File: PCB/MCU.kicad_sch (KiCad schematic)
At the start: 12 parts, among them J1 TC2030-NL, U7 STM32G431C8Ux

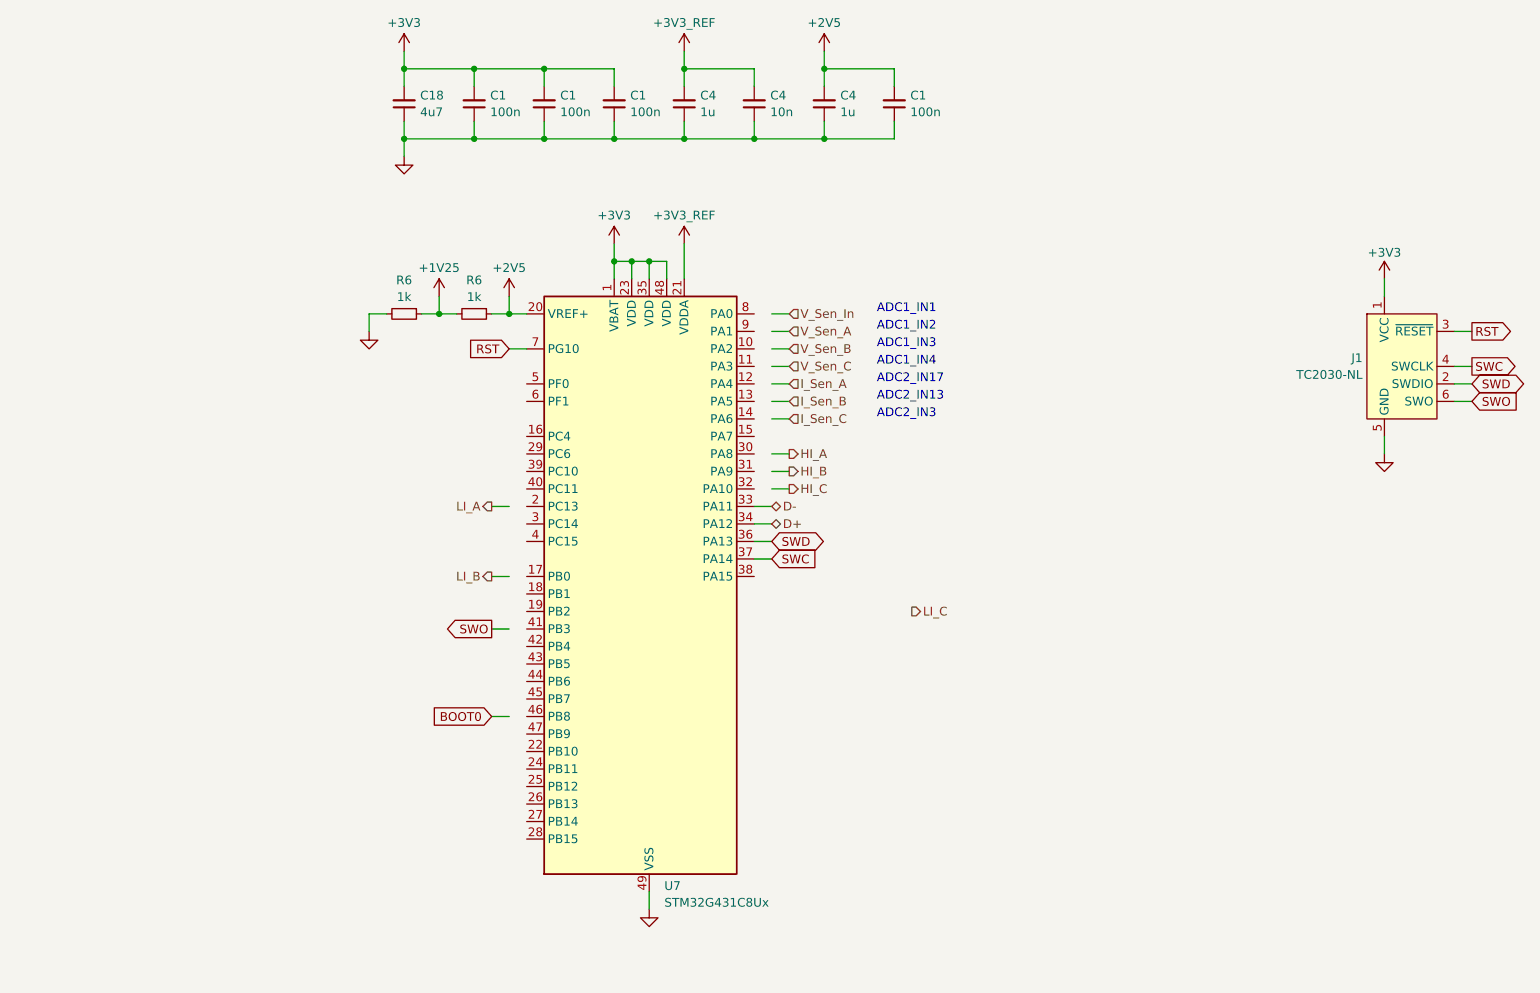
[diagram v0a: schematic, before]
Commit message: f
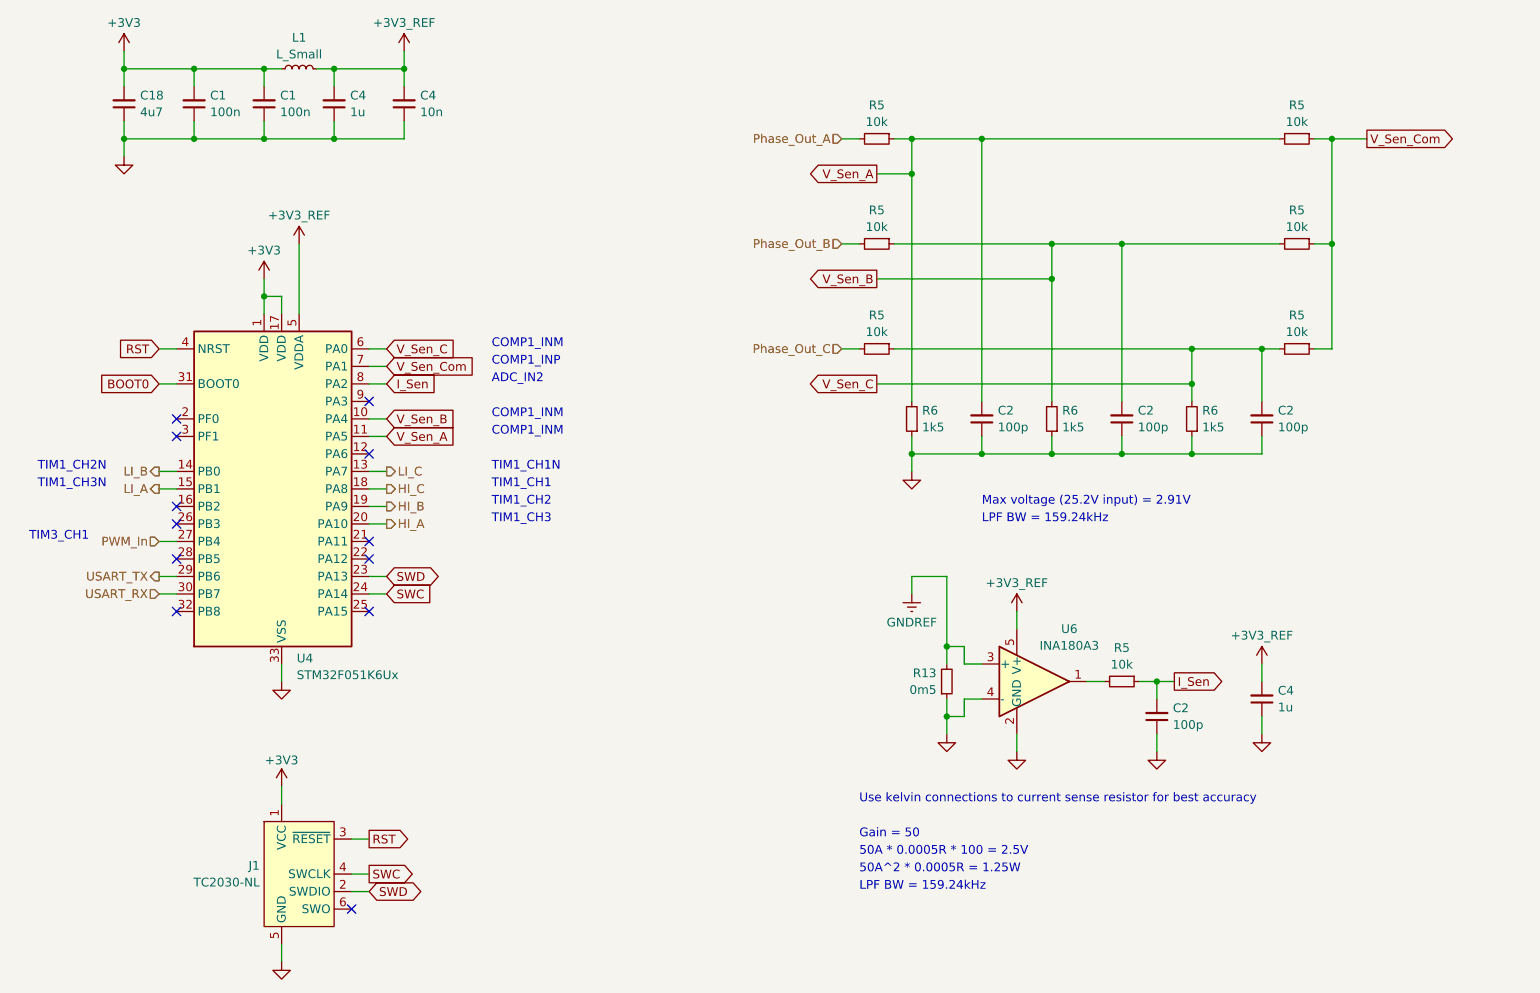
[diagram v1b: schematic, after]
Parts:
- removed C1 (x2): 100n, symbol Device:C_Small
- removed R6 (x2): 1k, symbol Device:R_Small
- removed U7: STM32G431C8Ux, Package_DFN_QFN:QFN-48-1EP_7x7mm_P0.5mm_EP5.6x5.6mm, symbol MCU_ST_STM32G4:STM32G431C8Ux
- added C2 (x4): 100p, symbol Device:C_Small
- added L1: L_Small, symbol Device:L_Small
- added R13: 0m5, symbol Device:R_Small
- added R5 (x7): 10k, symbol Device:R_Small
- added R6 (x3): 1k5, symbol Device:R_Small
- added U4: STM32F051K6Ux, Package_DFN_QFN:QFN-32-1EP_5x5mm_P0.5mm_EP3.45x3.45mm, symbol MCU_ST_STM32F0:STM32F051K6Ux
- added U6: INA180A3, Package_TO_SOT_SMD:SOT-23-5, symbol Amplifier_Current:INA180A3
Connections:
- net +2V5 is gone; now on net +3V3_REF: C4.2
- net +3V3: now also L1.1, U4.1 (VDD), U4.17 (VDD)
- net +3V3_REF: now also L1.2, U4.5 (VDDA), U6.5 (V+)
- net BOOT0: now also U4.31 (BOOT0)
- net GND: now also C2.1, C2.1, C2.1, C2.1, R13.1, R6.1, R6.1, R6.1, U4.33 (VSS), U6.2 (GND), U6.4 (-)
- net HI_A: now also U4.20 (PA10)
- net HI_B: now also U4.19 (PA9)
- net HI_C: now also U4.18 (PA8)
- net LI_A: now also U4.15 (PB1)
- net LI_B: now also U4.14 (PB0)
- net LI_C: now also U4.13 (PA7)
- net RST: now also U4.4 (NRST)
- net SWC: now also U4.24 (PA14)
- net SWD: now also U4.23 (PA13)
- net V_Sen_A: now also C2.2, R5.1, R5.2, R6.2, U4.11 (PA5)
- net V_Sen_B: now also C2.2, R5.1, R5.2, R6.2, U4.10 (PA4)
- net V_Sen_C: now also C2.2, R5.1, R5.2, R6.2, U4.6 (PA0)
- net SWO: no longer names the net of J1.6 (SWO)
- new net: R5.2, U6.1
- new net GNDREF: R13.2, U6.3 (+)
- new net I_Sen: C2.2, R5.1, U4.8 (PA2)
- new net PWM_In: U4.27 (PB4)
- new net Phase_Out_A: R5.2
- new net Phase_Out_B: R5.2
- new net Phase_Out_C: R5.2
- new net USART_RX: U4.30 (PB7)
- new net USART_TX: U4.29 (PB6)
- new net V_Sen_Com: R5.1, R5.1, R5.1, U4.7 (PA1)
- no-connect marks 0 -> 12
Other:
- note added: "50A * 0.0005R * 100 = 2.5V"
- note added: "50A^2 * 0.0005R = 1.25W"
- note added: "ADC_IN2"
- note added: "COMP1_INM"
- note added: "COMP1_INP"
- note added: "Gain = 50"
- note added: "LPF BW = 159.24kHz"
- note added: "Max voltage (25.2V input) = 2.91V"
- note added: "TIM1_CH1"
- note added: "TIM1_CH1N"
- note added: "TIM1_CH2"
- note added: "TIM1_CH2N"
- note added: "TIM1_CH3"
- note added: "TIM1_CH3N"
- note added: "TIM3_CH1"
- note added: "Use kelvin connections to current sense resistor for best accuracy"
- note removed: "ADC1_IN1"
- note removed: "ADC1_IN2"
- note removed: "ADC1_IN3"
- note removed: "ADC1_IN4"
- note removed: "ADC2_IN13"
- note removed: "ADC2_IN17"
- note removed: "ADC2_IN3"
- moved on the sheet: C1, C18, C4, J1
